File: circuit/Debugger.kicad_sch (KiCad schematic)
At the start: 2 parts

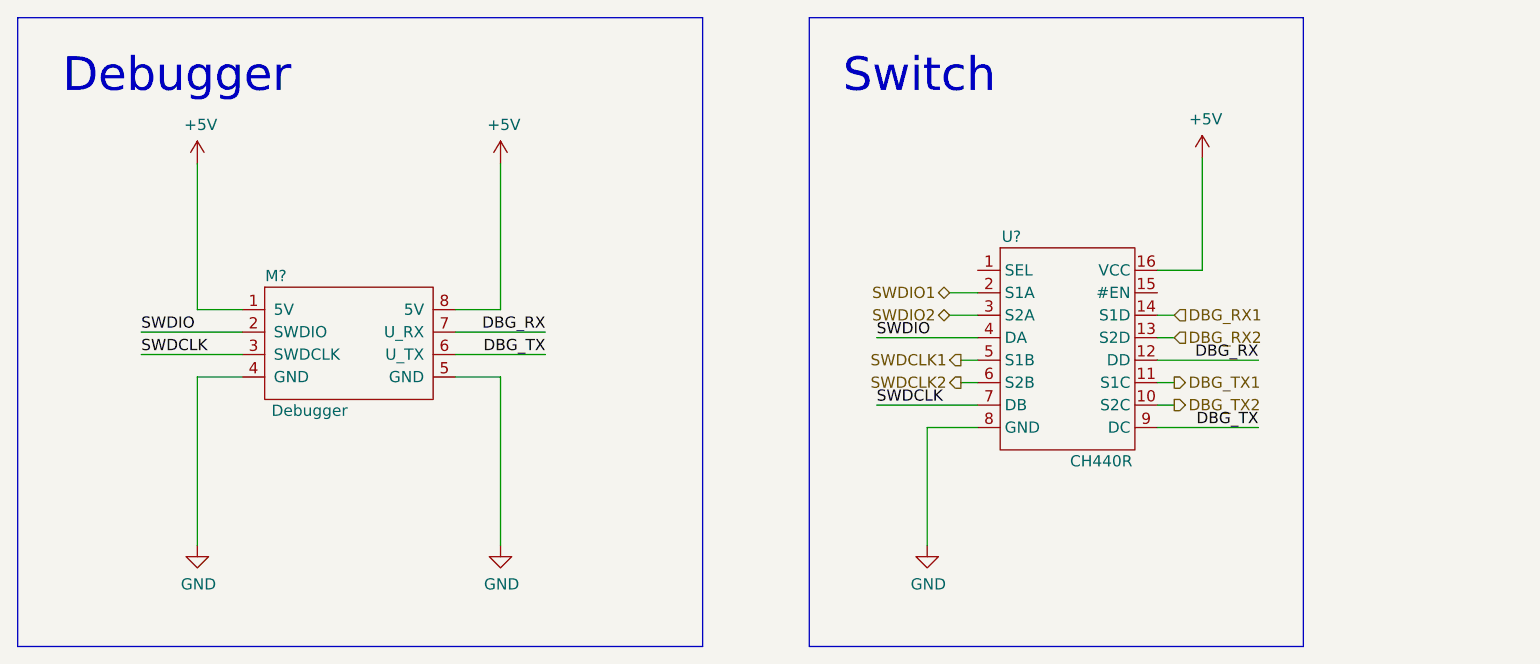
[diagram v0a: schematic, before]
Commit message: Basically finished schematic drawing and annotation, not yet package selection.
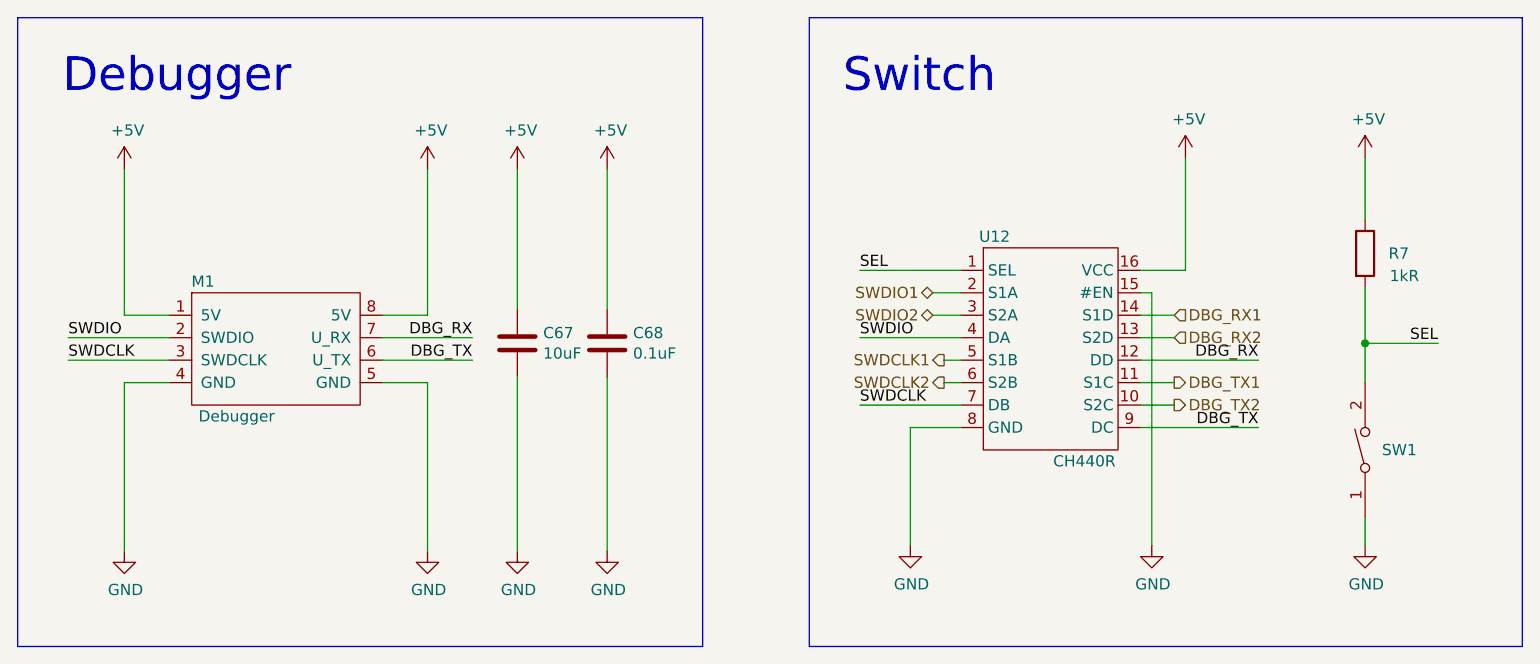
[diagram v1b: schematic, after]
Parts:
- added C67: 10uF, Capacitor_SMD:C_0603_1608Metric, symbol Device:C
- added C68: 0.1uF, Capacitor_SMD:C_0603_1608Metric, symbol Device:C
- added R7: 1kR, Resistor_SMD:R_0603_1608Metric, symbol Device:R
- added SW1: SW_DIP_x01, symbol Switch:SW_DIP_x01
- gave numbers to parts that had none: 2
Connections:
- net +5V: now also C67.1, C68.1, R7.1
- net GND: now also U12.15 (#EN), C67.2, C68.2, SW1.1
- net SEL: now reaches U12.1 (SEL)
- net SEL: now also R7.2, SW1.2
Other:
- moved on the sheet: M1, U12
